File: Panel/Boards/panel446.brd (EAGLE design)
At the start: 76.2 x 63.5 mm, 69 parts, among them IC101 STM32F446RET6, IC201 LM2596S-5V, IC202 LM1117-3V3, IC301 RS485SOIC, IC302 MCP2561-E/SN, IC303 MAX2021, IC304 TS5V330CDR, J201 JP_5V, J401 PANEL, J402 SONY, J403 THERMAL_DALI_VIDEO, J404 LRF_NOPTEL, J405 IMU, J406 PROG_DEBUG, Q101 8MHz, Q201 A03401, Q202 2N2222

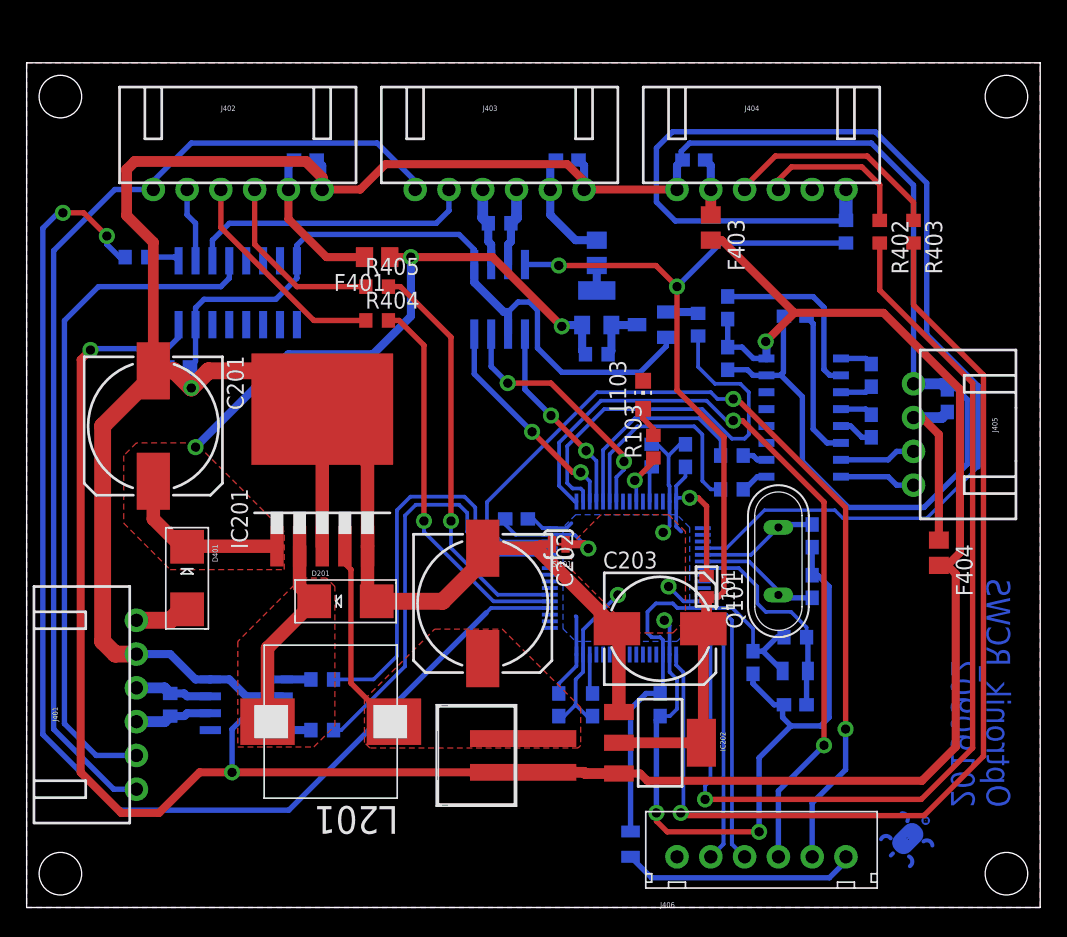
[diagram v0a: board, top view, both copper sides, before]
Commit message: v2.1.0
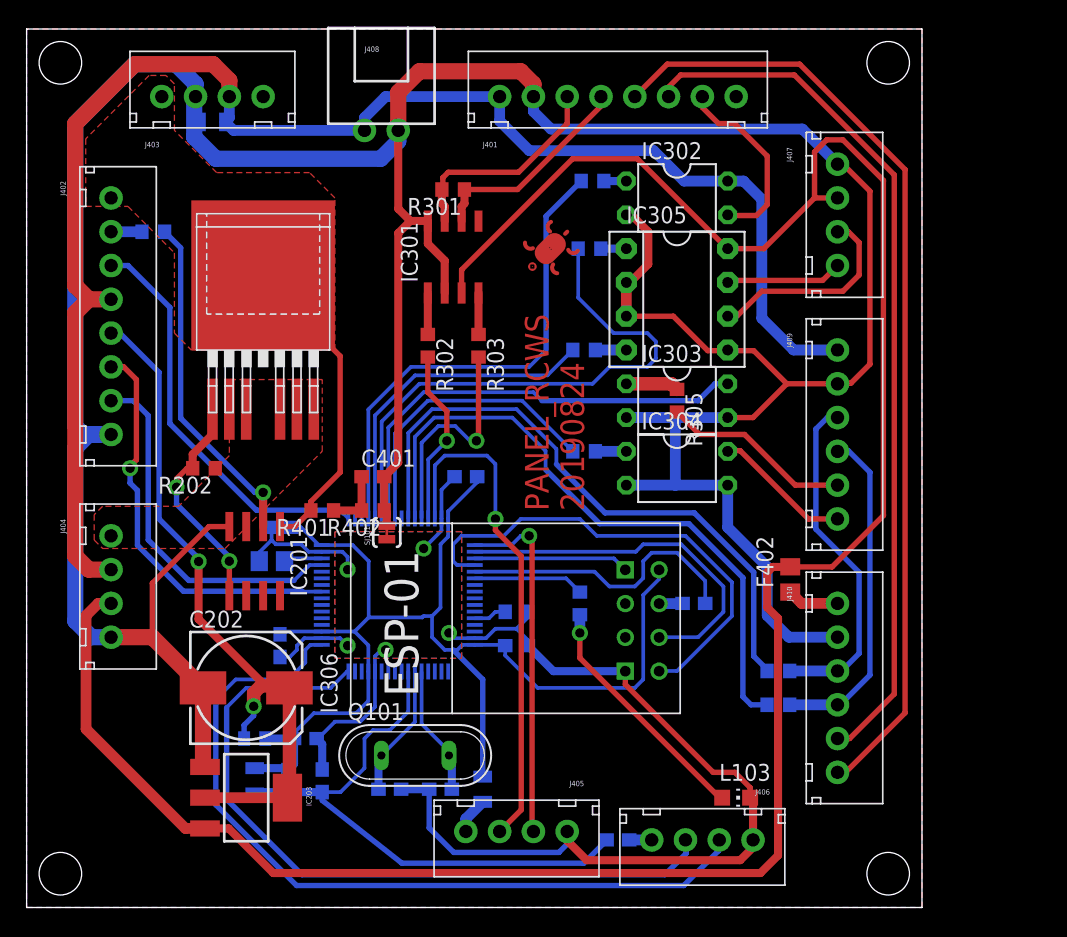
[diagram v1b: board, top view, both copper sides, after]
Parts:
- removed C201: 470u/35V, resistor:153CLV-1012
- removed C203: 1000u/6V3, resistor:153CLV-0810
- removed C302, C303, C304, C305, C306, C403, C404: 100n, resistor:C0603
- removed D201: SS34, adafruit:SMADIODE
- removed F401, F403, F404: 500mA, rcl:L0805
- removed J201: JP_5V, SparkFun-Connectors:XH-2-VERT-SMD
- removed L201: 33uH, scorpion:PA4342
- removed Q201: A03401, scorpion:SOT23-W
- removed Q202: 2N2222, scorpion:SOT23
- removed R203: 10k, resistor:R0603
- removed R204, R403, R404: 120R, resistor:R0603
- added IC203: LM1117-3V3, SparkFun:SOT223
- added IC305: MAX485DIL, SparkFun:DIL08
- added IC306: ESP01, esp8266modules:ESP01
- added J407: GPS, SparkFun-Connectors:XH-4-VERT
- added J408: PWR_MONITOR, SparkFun-Connectors:XH-2-RA
- added J409: PC, SparkFun-Connectors:XH-6-VERT
- added J410: SIGHTLINE, SparkFun-Connectors:XH-6-VERT
- added R201: 1k, rcl:R0603
- added R202: 100k, rcl:R0603
- added R308, R406: 120R, rcl:R0603
- C109: device resistor:C0603 -> rcl:C0805
- C202: value 470u/35V -> 1000u/6V3; device resistor:153CLV-1012 -> resistor:153CLV-0810
- C301: device rcl:C0603 -> resistor:C0603
- D401: value SS34 -> SCHOTTKY; device adafruit:SMADIODE -> diode:MICROMELF-W
- IC201: value LM2596S-5V -> MIC5014YM; device ON Semiconductor_By_element14_Batch_1:D2PAK -> microchip:SO-08
- IC202: value LM1117-3V3 -> IPB160; device SparkFun:SOT223 -> infineon:PG-TO263-7
- IC301: value RS485SOIC -> MCP2561-E/SN; device SparkFun-DigitalIC:SO08 -> microchip:SOIC-8
- IC302: value MCP2561-E/SN -> PC817-DIL; device microchip:SOIC-8 -> optocoupler:DIL04A
- IC303: value MAX2021 -> PC817-DIL; device SparkFun-DigitalIC:SO016 -> optocoupler:DIL04A
- IC304: value TS5V330CDR -> PC817-DIL; device Texas Instruments_By_element14_Batch_1:SOIC127P600X175-16N -> optocoupler:DIL04A
- J401: value PANEL -> BUS; device SparkFun-Connectors:XH-6-RA -> SparkFun-Connectors:XH-8-VERT
- J402: value SONY -> BUTTON; device SparkFun-Connectors:XH-6-RA -> SparkFun-Connectors:XH-8-VERT
- J403: value THERMAL_DALI_VIDEO -> POWER; device SparkFun-Connectors:XH-6-RA -> SparkFun-Connectors:XH-4-VERT
- J404: value LRF_NOPTEL -> DC CONVERTER; device SparkFun-Connectors:XH-6-RA -> SparkFun-Connectors:XH-4-VERT
- J405: value IMU -> PROG; device SparkFun-Connectors:XH-4-RA -> SparkFun-Connectors:XH-4-VERT
- J406: value PROG_DEBUG -> DEBUG; device SparkFun-Connectors:XH-6-VERT -> SparkFun-Connectors:XH-4-VERT
- R305, R306: value 120R -> 330R
- R401, R405: device resistor:R0603 -> rcl:R0603
- R402: value 120R -> 1k; device resistor:R0603 -> rcl:R0603
- moved J401 58.3 mm to (44.5, 61.0), turned to 0 degrees
- moved J404 57.3 mm to (6.35, 24.1), turned to 270 degrees
- moved U$1 51.9 mm to (39.4, 49.5), flipped to the bottom, turned to 270 degrees
- moved C402 51.3 mm to (44.5, 5.08)
- moved IC302 50.0 mm to (48.9, 53.3), flipped to the top
- moved R304 46.0 mm to (42.5, 54.6), turned to 0 degrees
- moved R401 44.6 mm to (22.2, 29.8), flipped to the top, turned to 180 degrees
- moved R402 43.5 mm to (26.0, 29.8), turned to 180 degrees
- moved C301 42.6 mm to (50.2, 22.9), turned to 0 degrees
- moved J405 42.2 mm to (36.8, 5.71), turned to 180 degrees
- moved IC202 42.0 mm to (17.8, 41.9), turned to 0 degrees
- moved R405 41.8 mm to (56.5, 17.8), flipped to the bottom
- moved D101 41.5 mm to (17.1, 9.53), turned to 270 degrees
- moved R102 39.6 mm to (19.7, 9.53), turned to 270 degrees
- moved C101 36.0 mm to (22.2, 9.53), turned to 90 degrees
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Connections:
- removed net !LRF_EN: IC101.4, J404.6, R401.2
- removed net CAM_SELECT: IC101.36, R307.2
- removed net IMU_RX: IC303.7, J405.3
- removed net IMU_RXD: IC101.53, R305.2
- removed net IMU_TX: IC303.8, J405.4
- removed net IMU_TXD: IC101.54, R306.2
- removed net LED: IC101.58, R103.1
- removed net LRF_RXD: IC101.16, R402.2
- removed net LRF_TXD: IC101.17, R403.2
- removed net N$1 (its old number): D402.A, J406.6
- removed net N$12: D401.A, J401.6
- removed net N$13: IC101.40
- removed net N$14: IC101.39
- removed net N$17 (its old number): Q202.1, R204.1
- removed net N$18 (its old number): IC302.4, R304.1
- removed net N$29 (its old number): C202.+, IC201.4, J201.2, L201.P$2
- removed net N$30: IC101.23
- removed net N$31 (its old number): C306.2, IC303.6
- removed net N$32: C303.2, IC303.1
- removed net N$33 (its old number): C304.2, IC303.4
- removed net N$39 (its old number): Q201.1, Q202.3, R203.2
- removed net N$43 (its old number): IC101.29
- removed net N$44 (its old number): IC101.33
- removed net N$47: C402.1, F402.1, J403.5
- removed net N$48: C403.1, F403.1, J404.2
- removed net N$5 (its old number): D201.C, IC201.2, L201.P$1
- removed net N$55: C404.1, F404.1, J405.2
- removed net N$72: C305.1, IC303.2
- removed net N$73: IC304.1, R307.1
- removed net N$74: IC303.10, R305.1
- removed net N$75: IC303.9, R306.1
- removed net RST: C101.1, D101.A, IC101.7, R102.2
- removed net SONY_RXD: IC101.37, R404.2
- removed net SONY_TXD: IC101.38, R405.2
- removed net SONY_VDD: C401.2, F401.2, J402.5
- removed net THERMAL_A: IC301.6, J403.3, R301.1
- removed net THERMAL_B: IC301.7, J403.4, R301.2
- removed net THERMAL_DE: IC101.55, IC301.3
- removed net THERMAL_PWR_EN: IC101.50, R204.2
- removed net THERMAL_RXD: IC101.51, IC301.4
- removed net THERMAL_TXD: IC101.52, IC301.1
- removed net THERMAL_VDD: F402.2, Q201.3
- removed net USART1_RXD: IC101.43
- removed net USART1_TXD: IC101.42
- removed net VIDEO_GND: J401.1, J402.1, J403.1
- removed net VIDEO_OUT: IC304.4, J401.2
- removed net VIDEO_SONY+: IC304.2, J402.2
- removed net VIDEO_THERMAL+: IC304.3, J403.2
- new net !RST: C101.1, C402.1, D101.A, IC101.7, R102.2
- new net BATT_VOLT: C401.1, IC101.23, R401.1, R402.2
- new net BUS_RESV: J401.8
- new net BUS_TRIGGER_PULSE: IC302.3, J401.7
- new net BUS_VIDEO+: J401.5, J410.6
- new net BUS_VIDEO-: J401.6, J410.5
- new net BUTTON_RXD: IC101.29, J402.7
- new net BUTTON_TXD: IC101.25, J402.6
- new net GATE: IC201.5, IC202.1, R202.2
- new net GPS_A_RX: IC305.6, J407.3
- new net GPS_B_TX: IC305.7, J407.4
- new net GPS_RXD: IC101.37, R308.2
- new net GPS_TXD: IC101.38, R307.2
- new net N$19: IC101.54, R103.1
- new net N$40: IC101.58
- new net N$41: IC101.55
- new net N$45: D402.A, J405.4
- new net N$46: IC301.4, R303.1
- new net N$57: IC101.14
- new net N$58: IC303.1, R305.1
- new net N$60: IC305.4, R308.1
- new net N$61: C402.2, J406.4
- new net N$65: F402.1, J410.1
- new net N$7: J409.3, J410.3, R405.1
- new net N$8: J409.4, J410.4, R406.1
- new net PC_IGNITE: IC304.4, J409.6
- new net PC_IGNITION: IC101.40, R306.2
- new net PC_PWR_CHECK: J409.5, R305.2
- new net PC_PWR_CHECK_IN: IC101.39, IC303.4
- new net PWR_BATT+: IC201.1, IC202.4, J402.1, J403.1, R401.2
- new net PWR_FROM_EMER: J402.2, R201.2
- new net PWR_RESV: J403.4
- new net PWR_TO_CONVERTER: IC201.3, IC202.2, IC202.3, IC202.5, IC202.6, IC202.7, J404.1, R202.1
- new net TRACKER_RXD: IC101.42, R405.2
- new net TRACKER_TXD: IC101.43, R406.2
- new net TRIGGER_IN: IC101.33, J402.3
- new net TRIG_PULSE_OUT: IC101.36, R304.2
- new net WIFI_EN: IC101.50, IC306.CH_PD
- new net WIFI_RST: C301.1, IC101.53
- new net WIFI_RXD: IC101.51, IC306.RX
- new net WIFI_TXD: IC101.52, IC306.TX
- net +12V: now also IC302.4, J401.1, J402.4, J403.3, J404.2, J408.1, J409.1; no longer C201.+, F401.1, IC201.1, Q201.2, R203.1
- net +3V3: now also C202.+, IC203.2, IC203.4, J402.5; no longer C203.+, IC202.2, IC202.4, IC301.8, R401.1
- net +5V: now also F402.2, IC203.3, IC301.3, IC305.8, J404.3, J407.2; no longer C301.1, C302.1, C305.2, F403.2, F404.2, IC202.3, IC302.3, IC303.16, IC304.16, J201.1
- net AGND: now also IC306.GND, J405.1, J406.1, L103.C
- net BUS_CANH: now also IC301.7, J401.3, R301.2; no longer IC302.7, J401.4, R302.2
- net BUS_CANL: now also IC301.6, J401.4, R301.1; no longer IC302.6, J401.3, R302.1
- net BUS_RXD: now also R303.2; no longer R304.2
- net BUS_TXD: now also R302.2; no longer R303.2
- net DEBUG_RXD: now also IC101.16; no longer IC101.14
- net DEBUG_TXD: now also IC101.17; no longer IC101.15
- net GND: now also C401.2, D401.A, IC201.4, IC203.1, IC301.8, IC303.2, IC303.3, IC304.2, IC304.3, IC305.2, IC305.3, IC305.5, J401.2, J402.8, J403.2, J404.4, J407.1, J408.2, J409.2, J410.2, R402.1; no longer C201.-, C203.-, C301.2, C302.2, C306.1, C401.1, C402.2, C403.2, C404.2, D201.A, IC201.3, IC201.5, IC201.6, IC202.1, IC301.5, IC302.8, IC303.15, IC304.15, IC304.8, J401.5, J402.6, J403.6, J404.1, J405.1, J406.1, L103.C, Q202.2
- net N$3: now also IC101.4; no longer J402.3, R404.1
- net N$49: now also IC301.1, R302.1; no longer IC302.1, R303.1
- net N$50: now also IC302.1, R304.1; no longer IC101.25
- net N$56: now also IC101.15; no longer J404.3, R403.1
- net N$59: now also IC305.1, R307.1; no longer J404.4, R402.1
- net N$68: now also IC304.1, R306.1; no longer C303.1, IC303.3
- net N$69: now also IC201.2, R201.1; no longer C304.1, IC303.5
- net N$9: now also C301.2, IC306.RST; no longer J402.4, R405.1
- net TCK: now also J405.2; no longer J406.4
- net TMS: now also J405.3; no longer J406.5
- net VDD: now also IC306.VCC
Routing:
- net CAM_SELECT: track 93.2 -> 0.00 mm, vias 2 -> 0
- net !LRF_EN: track 90.3 -> 0.00 mm
- net LRF_TXD: track 77.7 -> 0.00 mm, vias 1 -> 0
- net VIDEO_GND: track 76.8 -> 0.00 mm
- net LRF_RXD: track 76.0 -> 0.00 mm, vias 1 -> 0
- net BUS_VIDEO+: track 0.00 -> 72.4 mm
- net BUS_VIDEO-: track 0.00 -> 65.8 mm
- net +12V: track 56.7 -> 117.5 mm, vias 3 -> 0
- net VIDEO_OUT: track 51.7 -> 0.00 mm
- net TRACKER_TXD: track 0.00 -> 48.2 mm
- net TRACKER_RXD: track 0.00 -> 46.7 mm
- net !RST: track 0.00 -> 42.8 mm
- net GPS_TXD: track 0.00 -> 42.0 mm
- net DEBUG_TXD: track 19.5 -> 60.4 mm
- net TRIG_PULSE_OUT: track 0.00 -> 37.2 mm
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- added copper zone on layer 1, net PWR_BATT+
- added copper zone on layer 1, net PWR_TO_CONVERTER
- removed copper zone on layer 1, net +12V
- removed copper zone on layer 1, net N$29 (its old number)
- removed copper zone on layer 1, net N$5 (its old number)
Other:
- board size 76.2 x 63.5 mm -> 67.3 x 66 mm
- board text added: "PANEL_RCWS 20190824"
- board text removed: "Optronik_RCWS 20190902"
